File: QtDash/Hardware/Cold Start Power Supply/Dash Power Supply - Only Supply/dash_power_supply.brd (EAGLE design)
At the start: 50.8 x 45.4 mm, 26 parts, among them IC2 LM3488, Q4 BSC027N04LSG

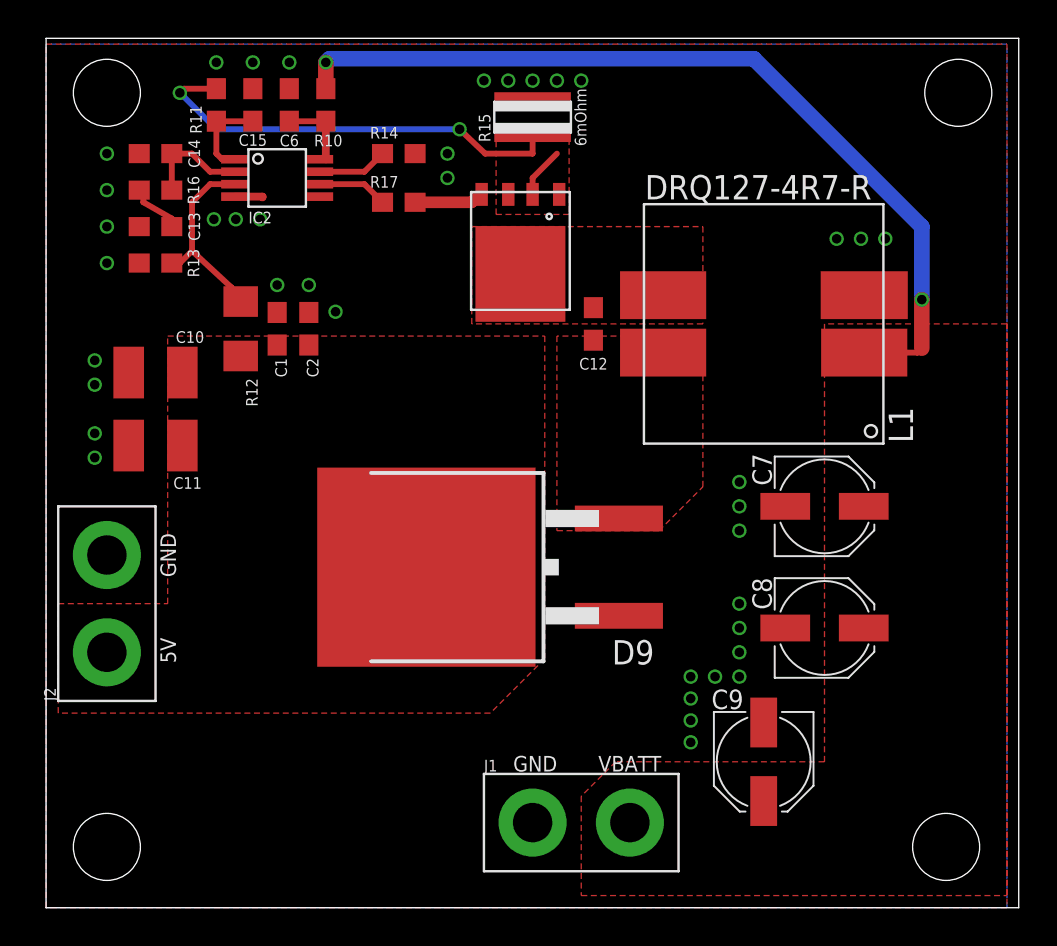
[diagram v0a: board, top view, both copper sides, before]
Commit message: topic/component-optimization: 	- rev b of cold start supply ordered
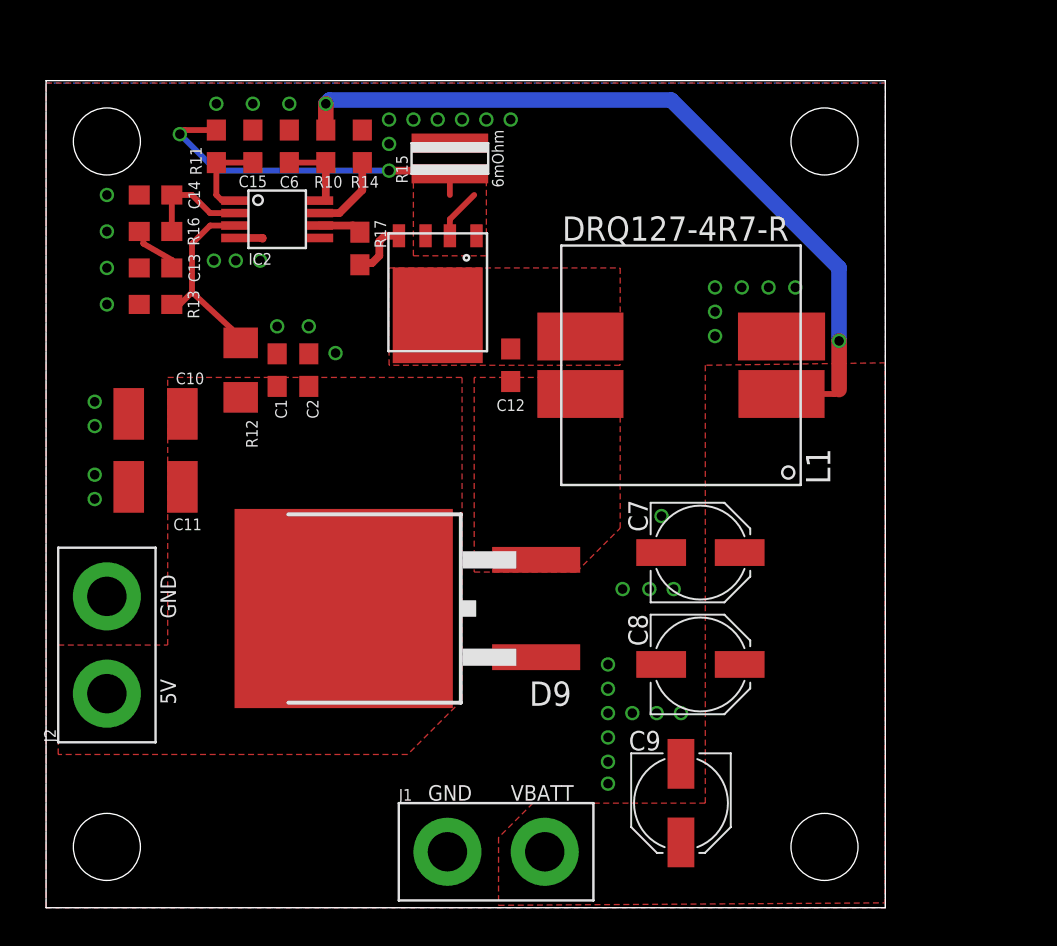
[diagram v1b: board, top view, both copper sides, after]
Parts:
- moved C7 6.91 mm to (34.2, 18.5)
- moved C8 6.75 mm to (34.2, 12.7)
- moved C9 4.83 mm to (33.1, 5.46)
- moved L1 4.83 mm to (33.1, 28.3)
- moved Q4 4.83 mm to (20.4, 32.1)
- moved D9 4.83 mm to (19.8, 15.6)
- moved C12 4.83 mm to (24.3, 28.3)
- moved R15 4.83 mm to (21.1, 39.1)
- moved J1 4.70 mm to (23.5, 2.92)
- moved R17 3.15 mm to (16.4, 34.4), turned to 270 degrees
- moved R16 2.16 mm to (5.71, 35.3)
- moved C10 2.16 mm to (5.71, 25.8)
- moved R13 2.16 mm to (5.71, 31.5)
- moved J2 2.16 mm to (3.17, 13.7)
- moved C1 2.16 mm to (12.1, 28.1)
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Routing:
- net N$17: track 25.5 -> 20.7 mm
- net VBATT: track 45.6 -> 41.3 mm
- net N$15: track 3.69 -> 2.26 mm
- net N$11: track 3.62 -> 3.11 mm
- net GND: vias 39 -> 43
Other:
- board size 50.8 x 45.4 mm -> 43.8 x 43.2 mm
- board text added: "Cold Start Power Supply VIN: 3-24V VOUT: 5.1V Rev B Mar 2022 @whitfijs"
